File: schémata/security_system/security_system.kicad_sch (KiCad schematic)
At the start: 12 parts

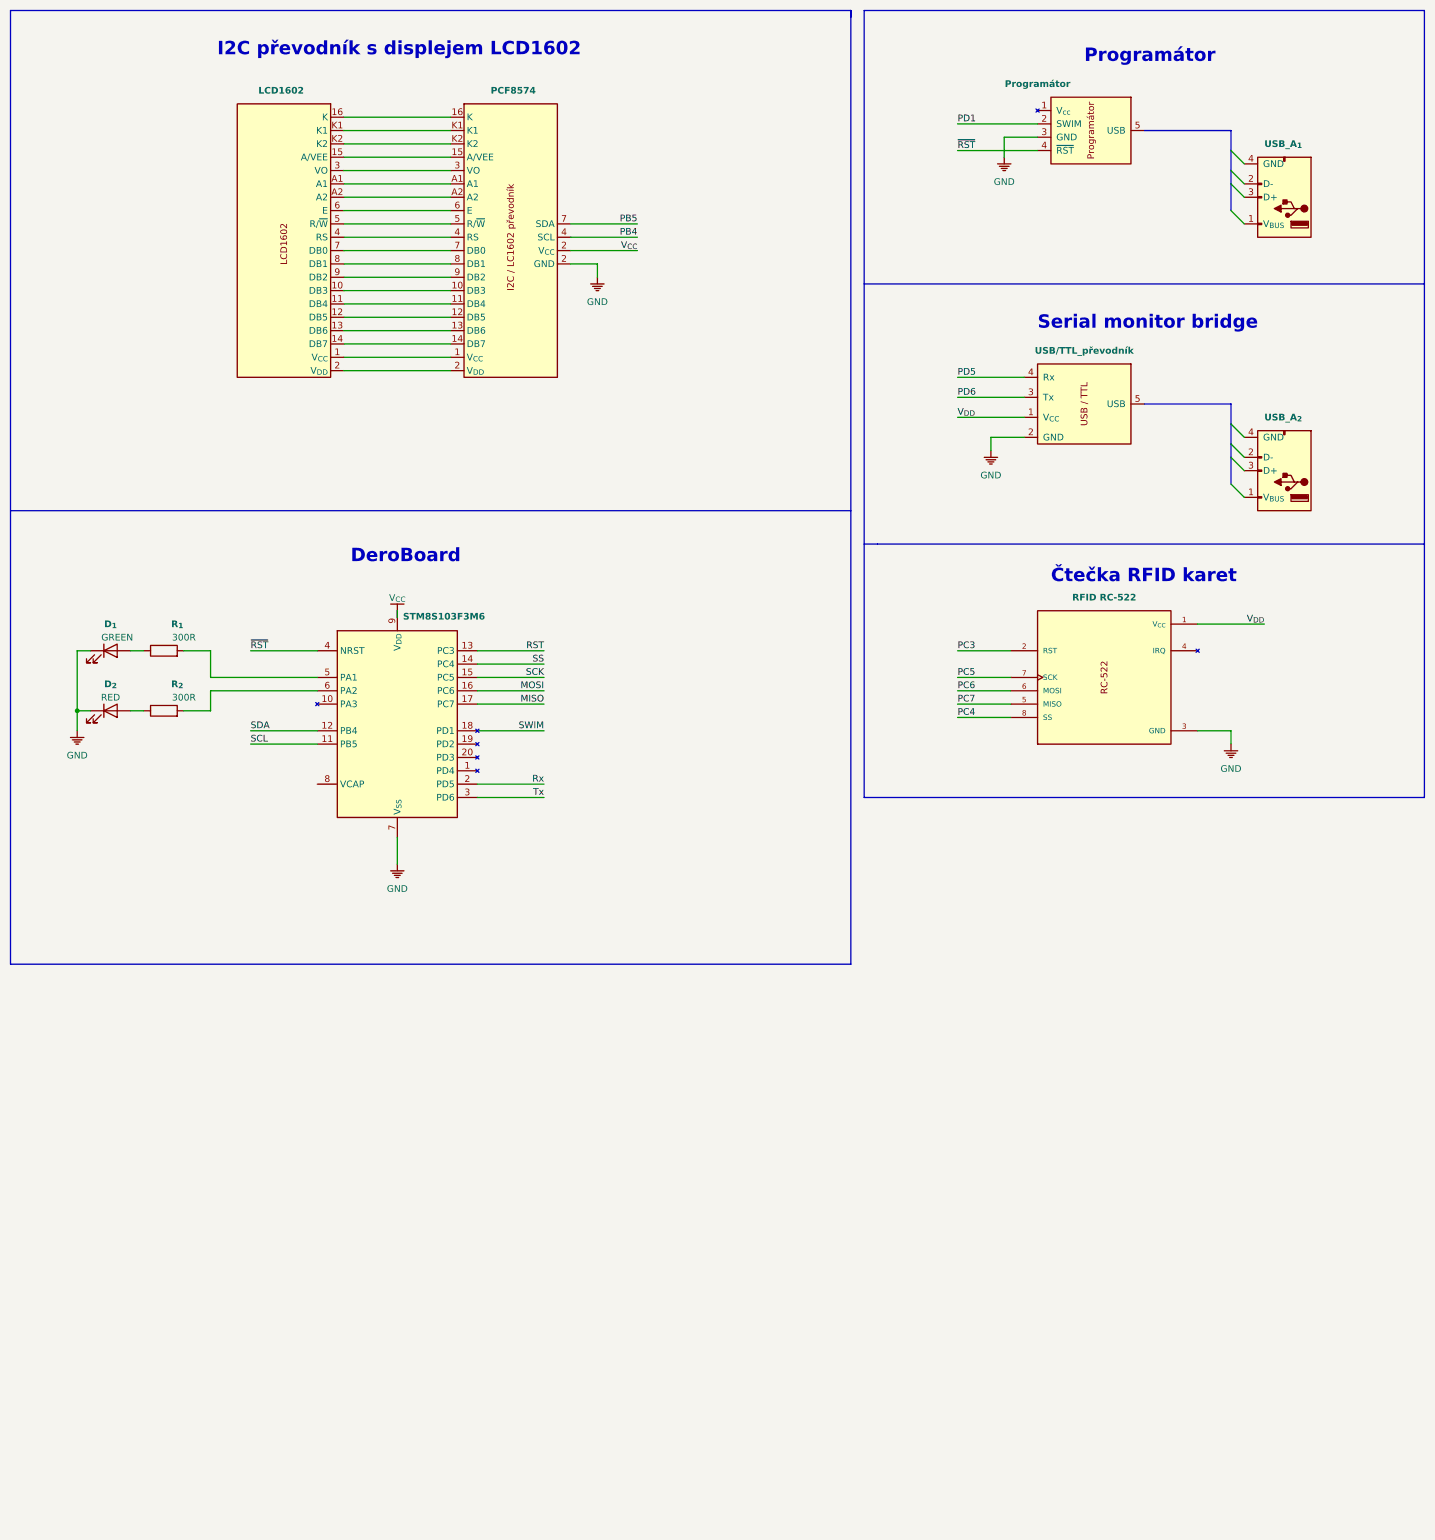
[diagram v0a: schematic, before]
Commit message: update
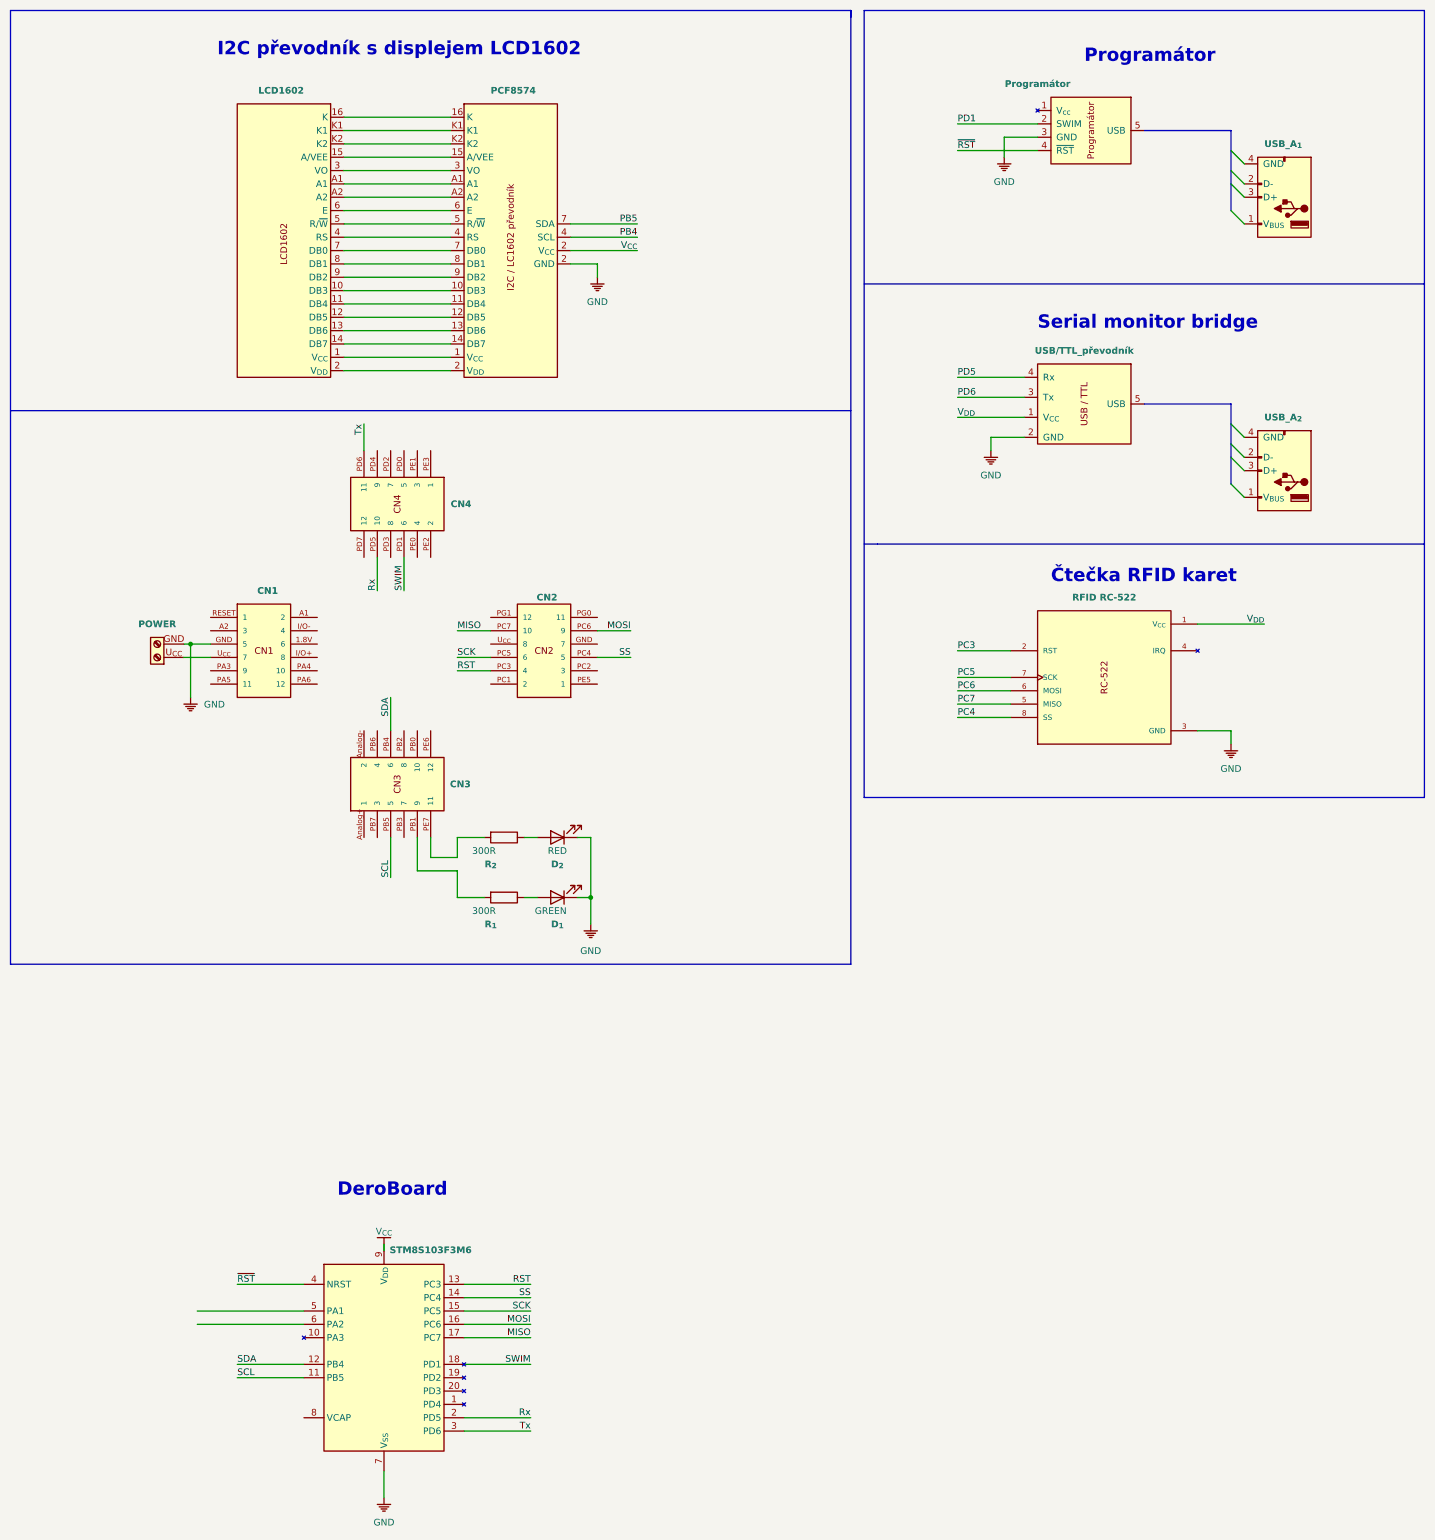
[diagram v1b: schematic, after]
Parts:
- removed U?: STM8S103F3M6, Package_SO:SO-20_12.8x7.5mm_P1.27mm, symbol KLIB_MCU_ST_STM8S:STM8S103F3M
- added CN1, CN2, CN3, CN4: 5-146258-6, Connector_PinSocket_2.54mm:PinSocket_2x06_P2.54mm_Vertical, symbol pin_header_2x12:5-146258-6
- added POWER: Screw_Terminal_01x02, symbol Connector:Screw_Terminal_01x02
- added U?: STM8S103F3M6, Package_SO:SO-20_12.8x7.5mm_P1.27mm, symbol KLIB_MCU_ST_STM8S:STM8S103F3M
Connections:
- net GND: now also CN1.GND (5), POWER.GND, U?.7 (V_{SS})
- net MISO: now also CN2.PC7 (10), U?.17 (PC7)
- net MOSI: now also CN2.PC6 (9), U?.16 (PC6)
- net RST: now also CN2.PC3 (4), U?.13 (PC3)
- net Rx: now also CN4.PD5 (10), U?.2 (PD5)
- net SCK: now also CN2.PC5 (6), U?.15 (PC5)
- net SCL: now also CN3.PB5 (5), U?.11 (PB5)
- net SDA: now also CN3.PB4 (6), U?.12 (PB4)
- net SS: now also CN2.PC4 (5), U?.14 (PC4)
- net SWIM: now also CN4.PD1 (6), U?.18 (PD1)
- net Tx: now also CN4.PD6 (11), U?.3 (PD6)
- net VDD: now also U?.9 (V_{DD})
- net ~{RST}: now also U?.4 (NRST)
- net at R_{1}.2: now also CN3.PB1 (9)
- net at R_{2}.2: now also CN3.PE7 (11)
- new net: CN1.U_{CC} (7), POWER.U_{CC} (Pin_1)
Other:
- moved on the sheet: D_{1}, D_{2}, R_{1}, R_{2}
